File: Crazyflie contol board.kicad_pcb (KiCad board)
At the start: 4 copper layers, 38.1 x 38.1 mm, 100 parts, among them P1 CONN_2, P2 CONN_2, P3 CONN_2, P4 CONN_2, P7 MICRO-B-USB, P9 CONN_1, Q1 PMV31XN, Q2 PMV31XN, Q3 PMV31XN, Q4 PMV31XN, Q5 2N7002, Q6 2N7002, Q7 SS8050-G, Q8 SS8050-G, SW1 PUSH ON/OFF, SW2 BOOT, U10 MAX16054, U11 ESP32-WROOM, U12 CP2102N-A01-GQFN24, U3 MPU60X0, U4 HMC5883L, U5 MS5611-01BA03, U6 NUF2221, U7 TPS79301, U8 BQ24075, U9 TPS79301

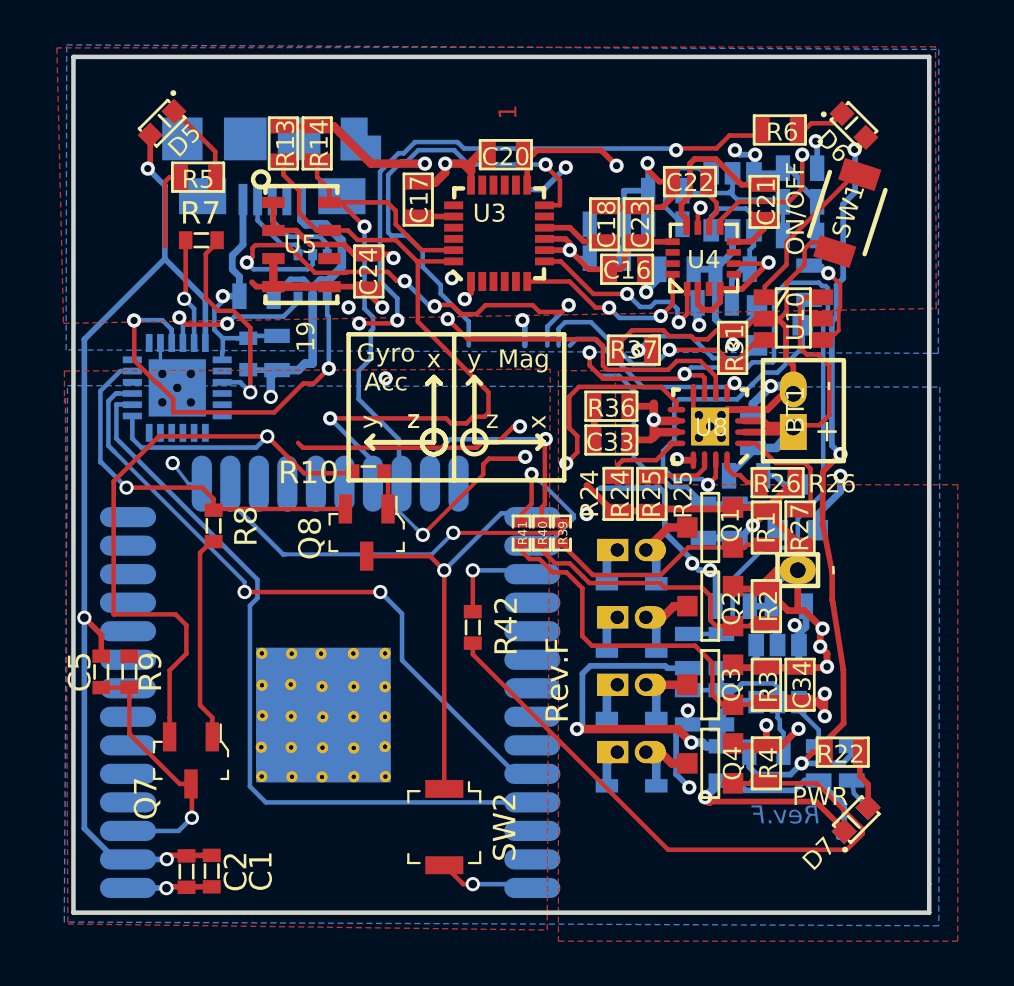
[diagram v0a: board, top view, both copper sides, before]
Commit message: version 2.0
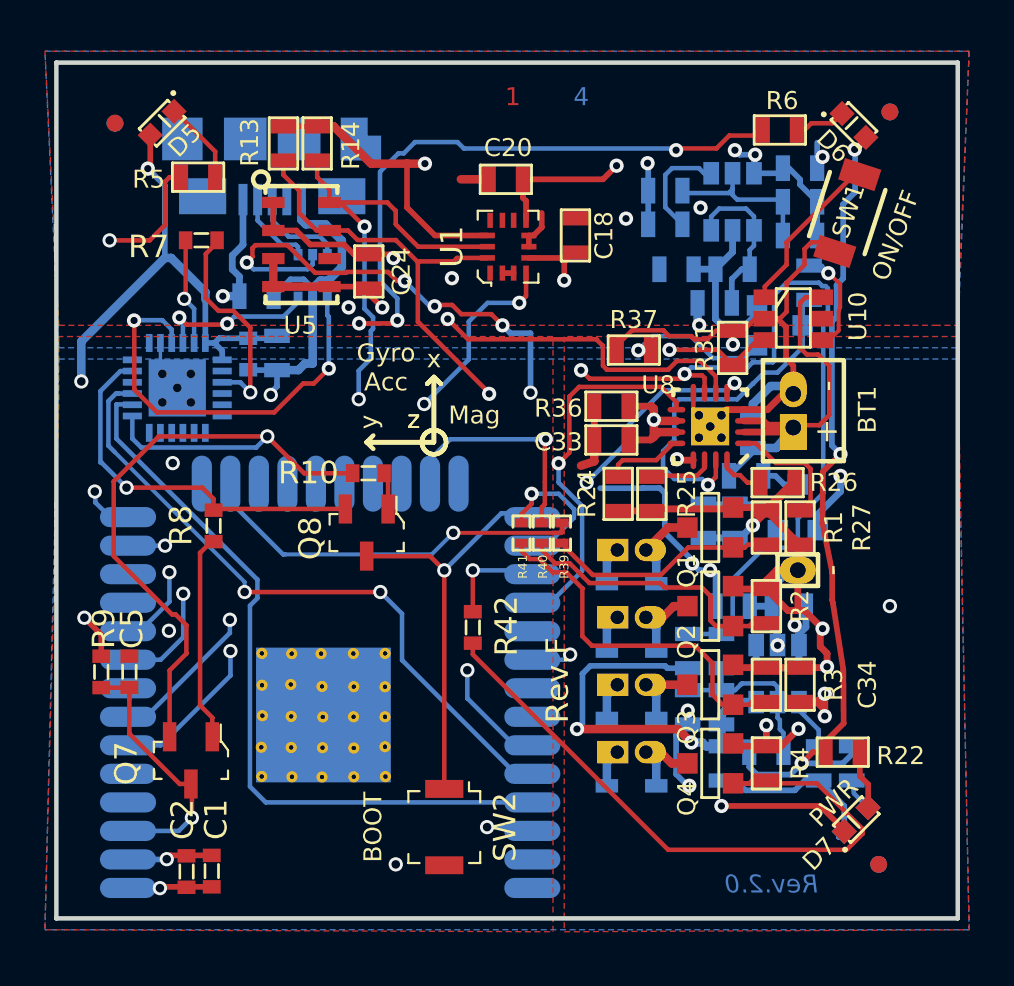
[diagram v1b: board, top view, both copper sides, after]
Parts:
- removed C16, C8: 10nF, SM0603_Capa
- removed C17: 2.2nF, SM0603_Capa
- removed C21: 0.22uF, SM0603_Capa
- removed C22, C7: 4.7uF, SM0603_Capa
- removed C23: 100nF, SM0603_Capa
- removed U3: MPU60X0, MPU60X0
- removed U4: HMC5883L, QFN16_HMC5883L
- added ?: Fiducial_0.75mm_Dia_1.5mm_Outer, Fiducials:Fiducial_0.75mm_Dia_1.5mm_Outer, B.Cu at (156.5, 118.5)
- added ?: Fiducial_0.75mm_Dia_1.5mm_Outer, Fiducials:Fiducial_0.75mm_Dia_1.5mm_Outer, B.Cu at (157.0, 85.0)
- added ?: Fiducial_0.75mm_Dia_1.5mm_Outer, Fiducials:Fiducial_0.75mm_Dia_1.5mm_Outer, B.Cu at (122.5, 85.5)
- added ?: Fiducial_0.75mm_Dia_1.5mm_Outer, Fiducials:Fiducial_0.75mm_Dia_1.5mm_Outer, F.Cu at (122.5, 85.5)
- added ?: Fiducial_0.75mm_Dia_1.5mm_Outer, Fiducials:Fiducial_0.75mm_Dia_1.5mm_Outer, F.Cu at (156.5, 118.5)
- added ?: Fiducial_0.75mm_Dia_1.5mm_Outer, Fiducials:Fiducial_0.75mm_Dia_1.5mm_Outer, F.Cu at (157.0, 85.0)
- added U1: BMX160, digikey-footprints:LGA-14L_2.5x3mm__LSM6DS3, F.Cu at (140.0, 91.0)
- moved C18 1.39 mm to (143.0, 90.5)
- moved C20 1.10 mm to (139.9, 88.0)
- turned C5 to 270 degrees
- turned R8 to 90 degrees
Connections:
- net /POWER/USBD+ renamed /USBD+
- net /POWER/USBD- renamed /USBD-
- C18 pad 1: Net-(C18-Pad1) -> VCCA
- C3 pad 2: /POWER/VUSB -> VCC
- C4 pad 2: /POWER/VUSB -> VCC
- C5 pad 1: Net-(C5-Pad1) -> DGND
- C5 pad 2: DGND -> Net-(C5-Pad2)
- P7 pad 4: Net-(P7-Pad4) -> (no net)
- Q7 pad 3: Net-(C5-Pad1) -> Net-(C5-Pad2)
- R5 pad 1: /LED_RED -> Net-(R5-Pad1)
- R6 pad 1: /LED_GREEN -> Net-(R6-Pad1)
- R8 pad 1: Net-(Q8-Pad2) -> Net-(Q7-Pad1)
- R8 pad 2: Net-(Q7-Pad1) -> Net-(Q8-Pad2)
- R9 pad 2: Net-(C5-Pad1) -> Net-(C5-Pad2)
- U10 pad 5: Net-(U10-Pad5) -> (no net)
- U11 pad 10: Net-(U11-Pad10) -> /EN1
- U11 pad 11: Net-(U11-Pad11) -> (no net)
- U11 pad 12: Net-(U11-Pad12) -> (no net)
- U11 pad 13: Net-(U11-Pad13) -> Net-(R6-Pad1)
- U11 pad 14: Net-(U11-Pad14) -> Net-(R5-Pad1)
- U11 pad 17: Net-(U11-Pad17) -> (no net)
- U11 pad 18: Net-(U11-Pad18) -> (no net)
- U11 pad 19: Net-(U11-Pad19) -> (no net)
- U11 pad 20: Net-(U11-Pad20) -> (no net)
- U11 pad 21: /I2C_SCK_VCCA -> (no net)
- U11 pad 22: /I2C_SCL_VCCA -> (no net)
- U11 pad 24: Net-(U11-Pad24) -> (no net)
- U11 pad 28: Net-(U11-Pad28) -> /CHG
- U11 pad 29: Net-(U11-Pad29) -> (no net)
- U11 pad 3: Net-(C5-Pad1) -> Net-(C5-Pad2)
- U11 pad 30: Net-(U11-Pad30) -> /PGOOD
- U11 pad 31: Net-(U11-Pad31) -> (no net)
- U11 pad 32: Net-(U11-Pad32) -> (no net)
- U11 pad 33: Net-(U11-Pad33) -> /I2C_SCK_VCCA
- U11 pad 36: Net-(U11-Pad36) -> /I2C_SCL_VCCA
- U11 pad 37: Net-(U11-Pad37) -> (no net)
- U11 pad 4: Net-(U11-Pad4) -> (no net)
- U11 pad 5: Net-(U11-Pad5) -> (no net)
- U11 pad 6: Net-(U11-Pad6) -> /EN2
- U11 pad 7: Net-(U11-Pad7) -> /SYSOFF
- U11 pad 8: Net-(U11-Pad8) -> (no net)
- U11 pad 9: Net-(U11-Pad9) -> /INT_GA
- U12 pad 1: Net-(U12-Pad1) -> (no net)
- U12 pad 10: Net-(U12-Pad10) -> (no net)
- U12 pad 11: Net-(U12-Pad11) -> (no net)
- U12 pad 12: Net-(U12-Pad12) -> (no net)
- U12 pad 13: Net-(U12-Pad13) -> (no net)
- U12 pad 14: Net-(U12-Pad14) -> (no net)
- U12 pad 15: Net-(U12-Pad15) -> (no net)
- U12 pad 16: Net-(U12-Pad16) -> (no net)
- U12 pad 17: Net-(U12-Pad17) -> (no net)
- U12 pad 18: Net-(U12-Pad18) -> (no net)
- U12 pad 22: Net-(U12-Pad22) -> (no net)
- U12 pad 24: Net-(U12-Pad24) -> (no net)
- U12 pad 7: /POWER/VUSB -> VCC
- U12 pad 8: Net-(U12-Pad8) -> (no net)
- U5 pad 6: Net-(U5-Pad6) -> (no net)
- U6 pad 5: /POWER/USB_CON -> VCC
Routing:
- net Net-(R6-Pad1): track 0.00 -> 42.5 mm, vias 0 -> 4
- net /EN2: track 8.98 -> 39.3 mm, vias 1 -> 3
- net /EN1: track 14.6 -> 43.2 mm, vias 1 -> 2
- net /SYSOFF: track 11.8 -> 40.4 mm, vias 1 -> 2
- net /LED_GREEN: track 27.0 -> 0.00 mm, vias 3 -> 0
- net AGND: track 40.3 -> 15.5 mm, vias 11 -> 6
- net /POWER/USB_CON: track 22.4 -> 0.00 mm, vias 4 -> 0
- net Net-(R5-Pad1): track 0.00 -> 19.1 mm, vias 0 -> 2
- net /PGOOD: track 36.3 -> 51.3 mm, vias 2 -> 3
- net Net-(C5-Pad2): track 0.00 -> 11.6 mm, vias 0 -> 1
- net Net-(C5-Pad1): track 11.6 -> 0.00 mm, vias 1 -> 0
- net /I2C_SCL_VCCA: track 32.5 -> 43.9 mm
- net Net-(U1-Pad16): track 10.4 -> 0.00 mm, vias 1 -> 0
- net Net-(U3-Pad7): track 9.23 -> 0.00 mm, vias 2 -> 0
- net Net-(U3-Pad6): track 8.73 -> 0.00 mm, vias 2 -> 0
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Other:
- board size 38.1 x 38.1 mm -> 40.1 x 38.1 mm
- board text added: "4"
- board text added: "BOOT"
- board text added: "Rev.2.0"
- board text removed: "19"
- board text removed: "R24"
- board text removed: "R25"
- board text removed: "R26"
